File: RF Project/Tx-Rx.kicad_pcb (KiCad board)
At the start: 2 copper layers, 30 x 55 mm, 26 parts, among them J1 CONN_Right, J2 CONN_Left, U1 CC2500RGPR, U2 U.FL_male

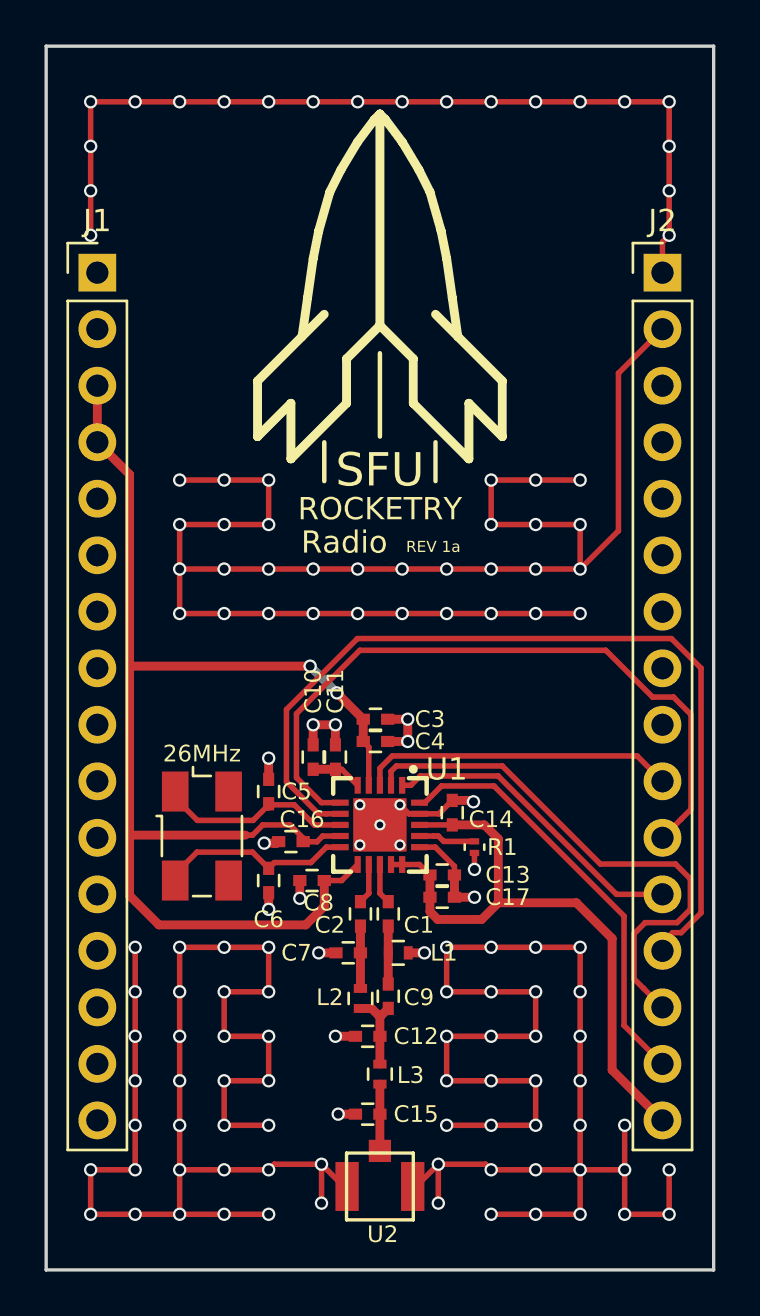
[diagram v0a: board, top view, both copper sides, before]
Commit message: Add files via upload
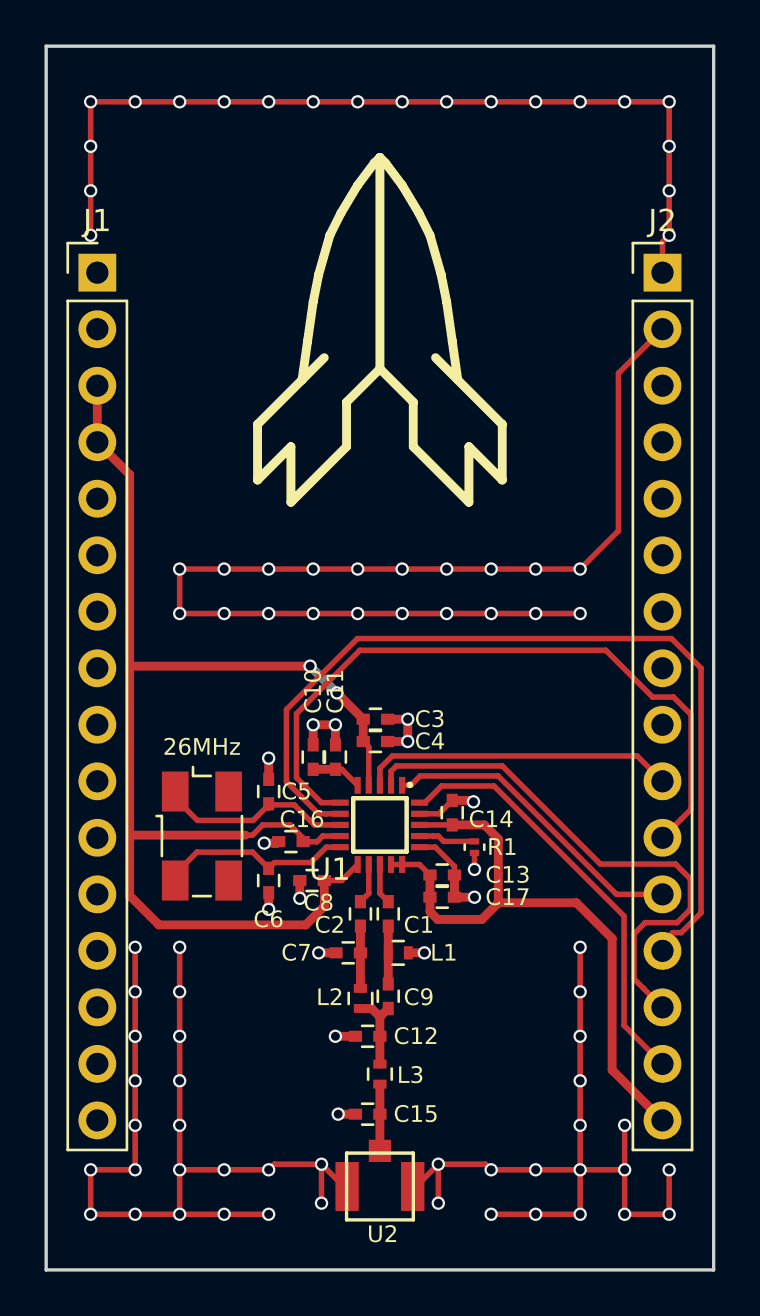
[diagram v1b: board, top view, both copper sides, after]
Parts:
- renumbered 26Mhtz1 to 26MHz
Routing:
- net PWR_GND: track 273.5 -> 190.0 mm, vias 137 -> 95
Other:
- board text removed: "26MHz"
- board text removed: "REV 1a"
- board text removed: "ROCKETRY"
- board text removed: "Radio"
- board text removed: "SFU"

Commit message: Resurrected kicad_pcb from the grave
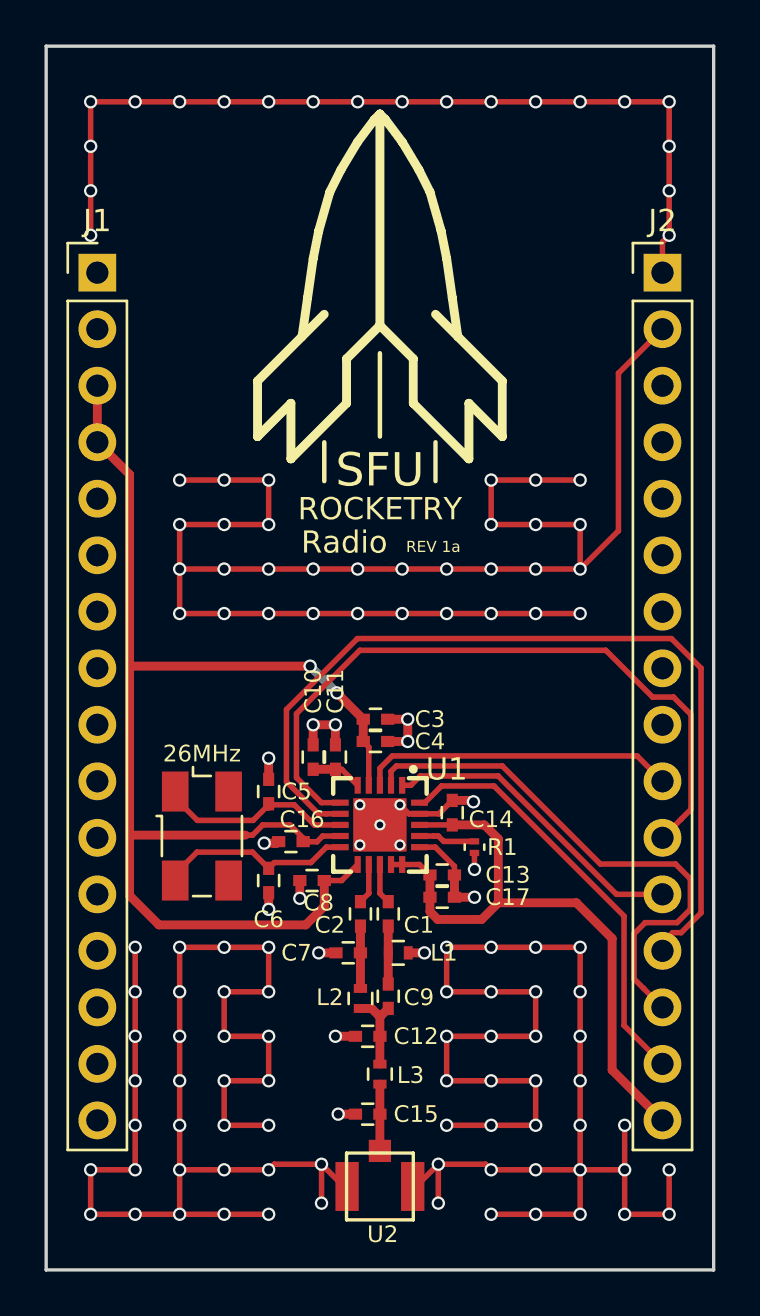
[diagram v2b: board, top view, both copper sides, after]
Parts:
- renumbered 26MHz to 26Mhtz1
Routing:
- net PWR_GND: track 190.0 -> 273.5 mm, vias 95 -> 137
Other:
- board text added: "26MHz"
- board text added: "REV 1a"
- board text added: "ROCKETRY"
- board text added: "Radio"
- board text added: "SFU"
